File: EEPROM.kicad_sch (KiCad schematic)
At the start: 22 parts, among them IC1 PCA6408A_TSSOP, IC2 AT24CS01_SOT23, U2 TPS613221A_SOT-23-5

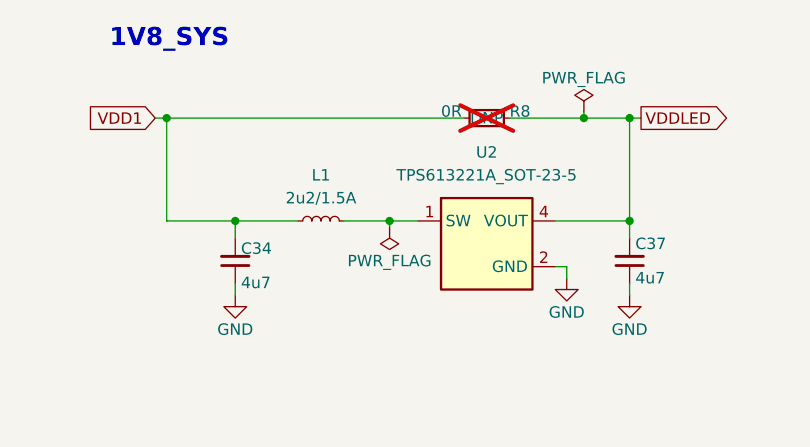
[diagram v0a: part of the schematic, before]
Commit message: [#86301] Project refresh 81589
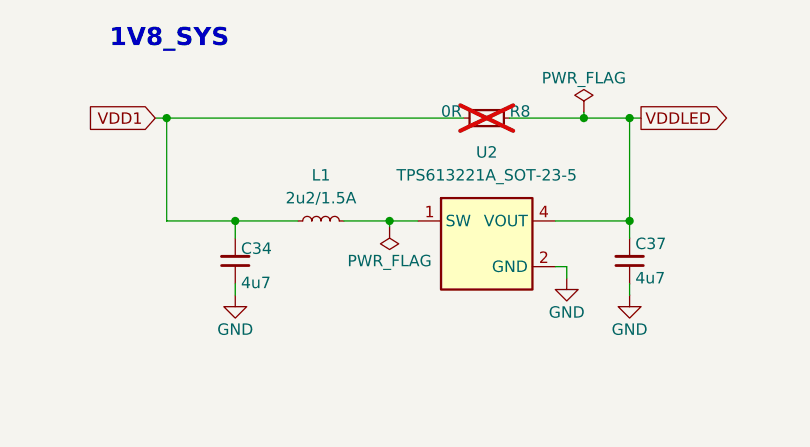
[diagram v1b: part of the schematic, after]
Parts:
- C34, C37: footprint lpddr4-testbed-footprints:C_0402_1005Metric -> antmicro-footprints:C_0402_1005Metric; symbol lpddr4-testbed:C_4u7_0402 -> antmicroCapacitors0402:C_4u7_0402
- C38, C39: footprint lpddr4-testbed-footprints:C_0402_1005Metric -> antmicro-footprints:C_0402_1005Metric; symbol lpddr4-testbed:C_100n_0402 -> antmicroCapacitors0402:C_100n_0402
- D1, D2, D3, D4: footprint lpddr4-testbed-footprints:LED_0603_1608Metric_G -> antmicro-footprints:LED_0603_1608Metric_G; symbol lpddr4-testbed:LED_G_0603_KP-1608CGCK -> antmicroLEDIndicationDiscrete:LED_G_0603_KP-1608CGCK
- IC1: footprint lpddr4-testbed-footprints:TSSOP-16_4.4x5mm_P0.65mm -> antmicro-footprints:TSSOP-16_4.4x5mm_P0.65mm; symbol lpddr4-testbed:PCA6408A_TSSOP -> antmicroInterfaceIOExpanders:PCA6408A_TSSOP
- IC2: footprint lpddr4-testbed-footprints:SOT-23-5 -> antmicro-footprints:SOT-23-5; symbol lpddr4-testbed:AT24CS01_SOT23 -> antmicroMemory:AT24CS01_SOT23
- L1: footprint lpddr4-testbed-footprints:L_0806_2016Metric -> antmicro-footprints:L_0806_2016Metric; symbol lpddr4-testbed:L_2u2_1.5A_0806 -> antmicroFixedInductors:L_2u2_1.5A_0806
- R10, R11, R12, R9: footprint lpddr4-testbed-footprints:R_0402_1005Metric -> antmicro-footprints:R_0402_1005Metric; symbol lpddr4-testbed:R_220R_0402 -> antmicroResistors0402:R_220R_0402
- R13, R14: footprint lpddr4-testbed-footprints:R_0402_1005Metric -> antmicro-footprints:R_0402_1005Metric; symbol lpddr4-testbed:R_10k_0402 -> antmicroResistors0402:R_10k_0402
- R8: footprint lpddr4-testbed-footprints:R_0402_1005Metric -> antmicro-footprints:R_0402_1005Metric; symbol lpddr4-testbed:R_0R_0402 -> antmicroResistors0402:R_0R_0402; DNP DNP -> (none)
- TP1, TP2, TP3: footprint lpddr4-testbed-footprints:TP_SMD_0.75mm -> antmicro-footprints:TP_SMD_0.75mm; symbol lpddr4-testbed:TP_0.75mm_SMD -> antmicroTestPoints:TP_0.75mm_SMD
- U2: footprint lpddr4-testbed-footprints:SOT-23-5 -> antmicro-footprints:SOT-23-5; symbol lpddr4-testbed:TPS613221A_SOT-23-5 -> antmicroDCDCConverters:TPS613221A_SOT-23-5
